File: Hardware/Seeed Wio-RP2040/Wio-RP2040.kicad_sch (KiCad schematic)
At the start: 23 parts, among them J1 USB_C_Receptacle_USB2.0, J2 Conn_01x06_Male, Q1 MMBT3904, Q2 MMBT3904, SW1 SW_Push, SW2 SW_DIP_x01, U1 CH340G, U2 AMS1117-3.3, Y1 12M

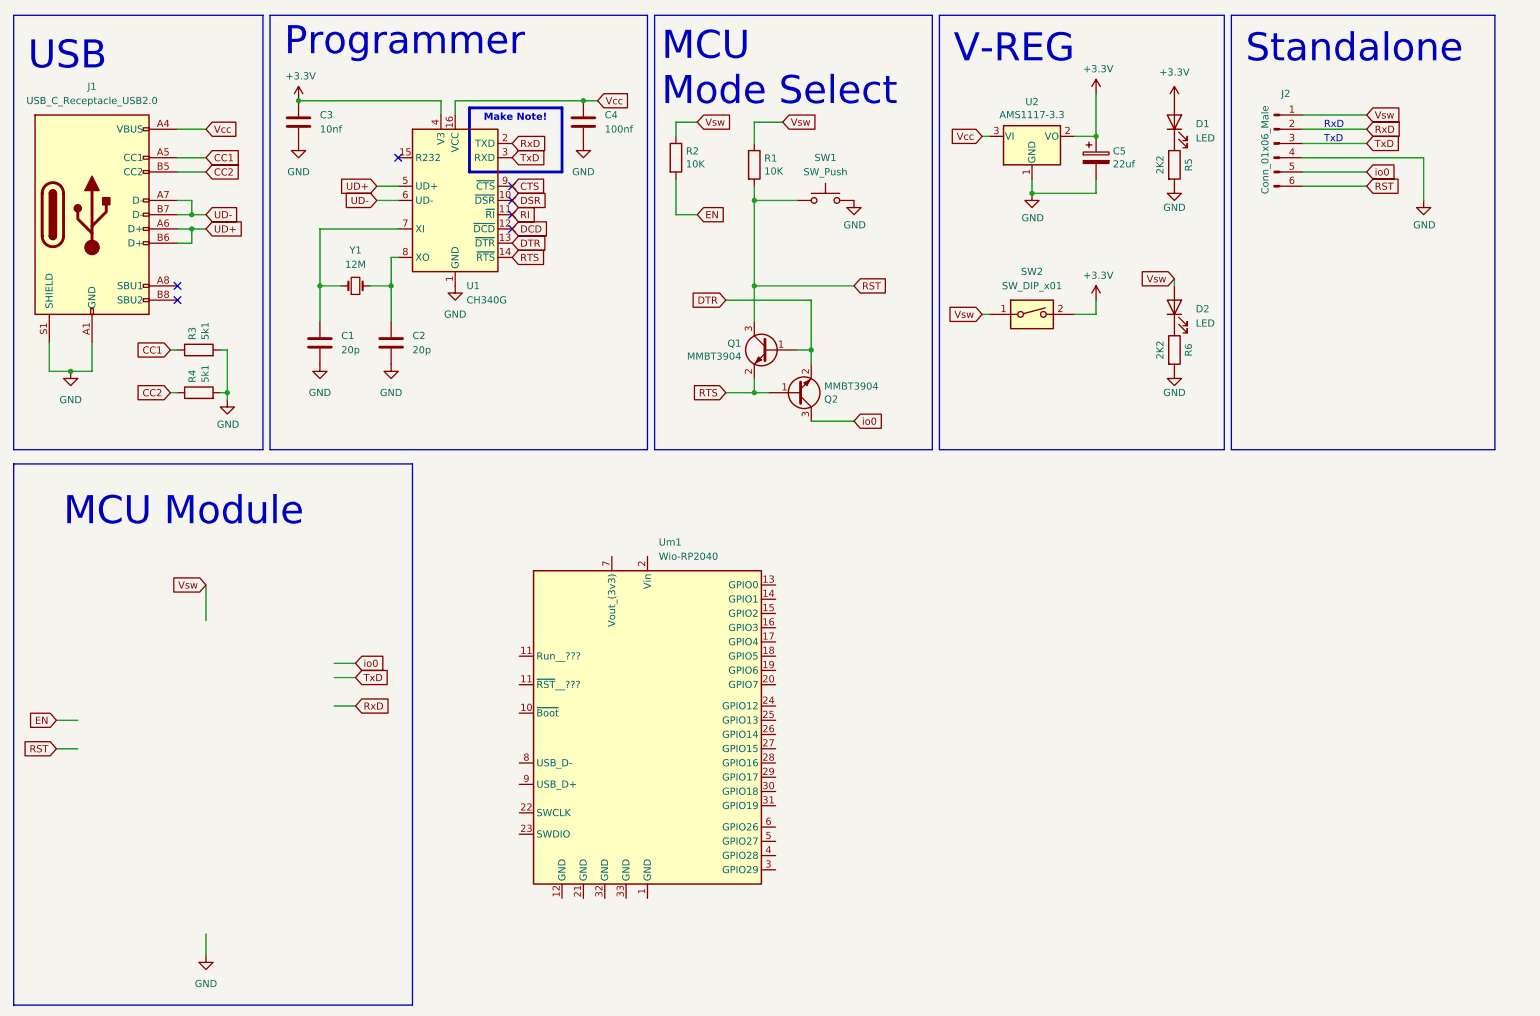
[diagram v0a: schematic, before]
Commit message: werkin on da RP2040
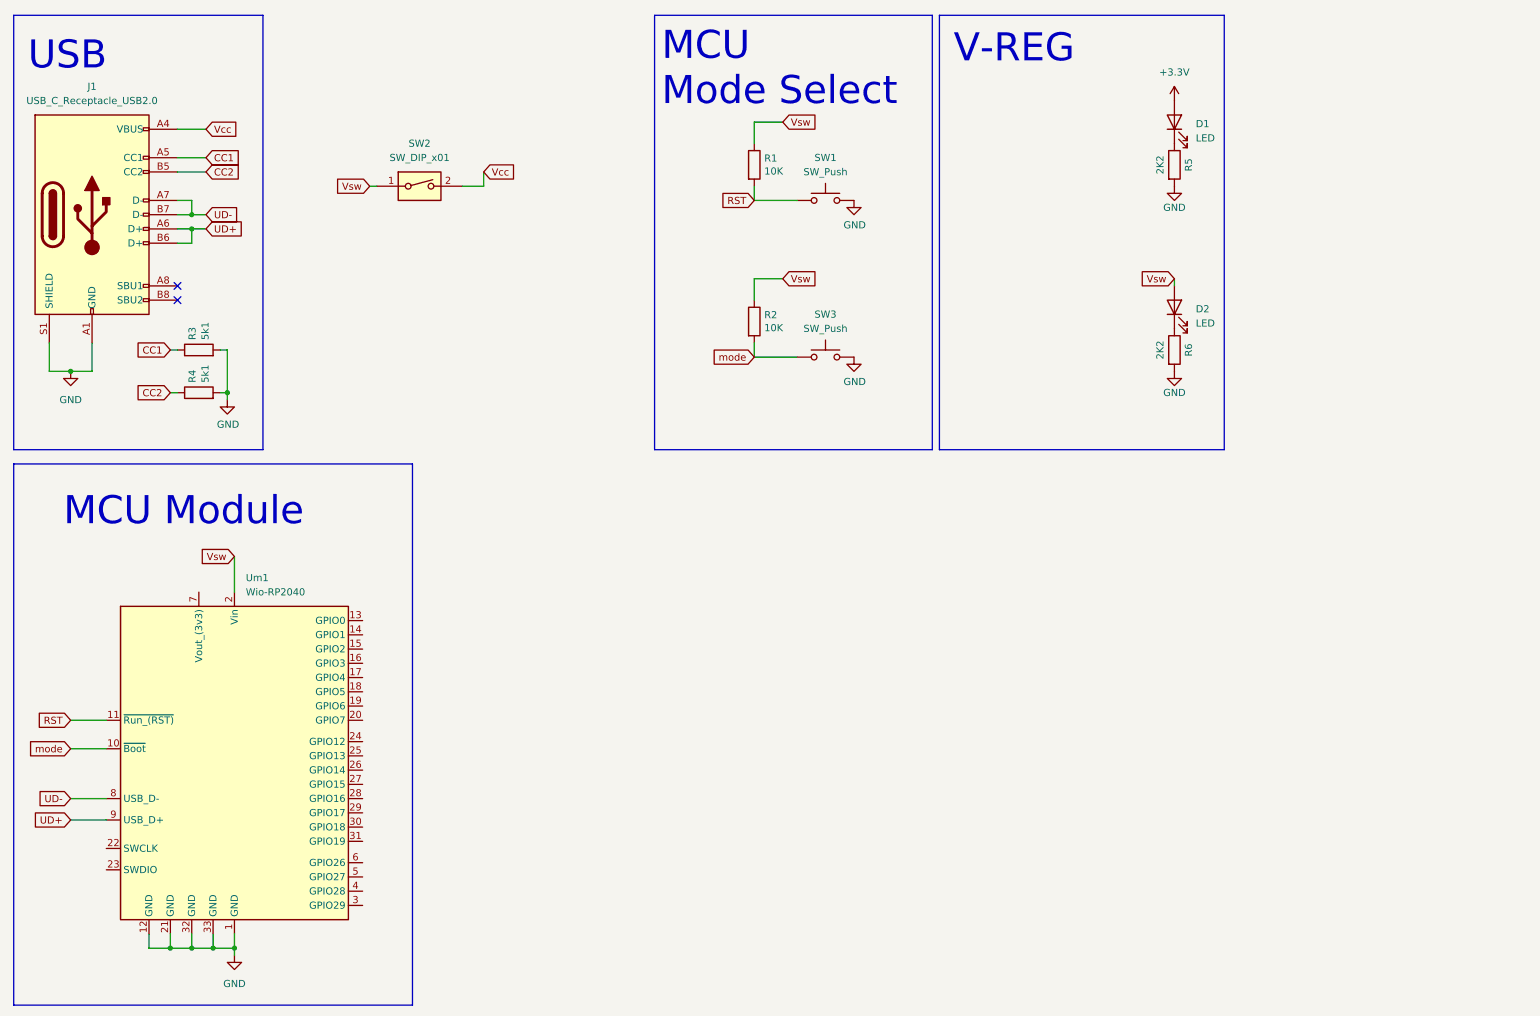
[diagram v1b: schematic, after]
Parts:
- removed C1, C2: 20p, Tinker:C_0603_1608Metric_Pad1.08x0.95mm_HandSolder, symbol Device:C
- removed C3: 10nf, Tinker:C_0603_1608Metric_Pad1.08x0.95mm_HandSolder, symbol Device:C
- removed C4: 100nf, Tinker:C_0603_1608Metric_Pad1.08x0.95mm_HandSolder, symbol Device:C
- removed C5: 22uf, Capacitor_Tantalum_SMD:CP_EIA-6032-28_Kemet-C_Pad2.25x2.35mm_HandSolder, symbol Device:CP
- removed J2: Conn_01x06_Male, Tinker:PinHeader_1x06_P2.54mm_Vertical, symbol Connector:Conn_01x06_Male
- removed Q1, Q2: MMBT3904, Package_TO_SOT_SMD:SOT-23_Handsoldering, symbol Transistor_BJT:MMBT3904
- removed U1: CH340G, Package_SO:SOIC-16_3.9x9.9mm_P1.27mm, symbol Interface_USB:CH340G
- removed U2: AMS1117-3.3, Package_TO_SOT_SMD:SOT-223-3_TabPin2, symbol Regulator_Linear:AMS1117-3.3
- removed Y1: 12M, Crystal:Crystal_SMD_5032-2Pin_5.0x3.2mm, symbol Device:Crystal_Small
- added SW3: SW_Push, Tinker:SW_Push_TS273014TP, symbol Switch:SW_Push
- D1, D2, R5, R6: now left out of the parts list
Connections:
- net EN is gone; now on net mode: R2.2
- net +3.3V: no longer SW2.2
- net GND: now also Um1.1 (GND), Um1.12 (GND), Um1.21 (GND), Um1.32 (GND), Um1.33 (GND), SW3.2
- net RST: now also Um1.11 (~{Run_(RST)})
- net UD+: now also Um1.9 (USB_D+)
- net UD-: now also Um1.8 (USB_D-)
- net Vcc: now also SW2.2
- net Vsw: now also Um1.2 (Vin)
- net mode: now reaches Um1.10 (~{Boot})
- net mode: now also SW3.1
- no-connect marks 7 -> 2
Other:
- note removed: "Make Note!"
- note removed: "Programmer"
- note removed: "RxD"
- note removed: "Standalone"
- note removed: "TxD"
- moved on the sheet: SW2
